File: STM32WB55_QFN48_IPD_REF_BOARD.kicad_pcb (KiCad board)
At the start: 4 copper layers, 72 parts, among them IC1 LD3985M33R, IC2 USBLC6-2SC6, J1 USB_B_Micro, J2 Conn_01x05_Male, J3 Conn_01x02_Male, J4 Conn_01x04_Male, J5 Conn_01x01_Male, J6 Conn_01x01_Male, J7 Conn_01x08_Male, U1 MCP1640CCH, U2 STM32WB55CG, U4 BNO055_my, U5 ADS1115IDGS, Y1 NX2520SA-32MHz, Y2 NX2012SA-32768K, Y3 NX2012SA-32768K

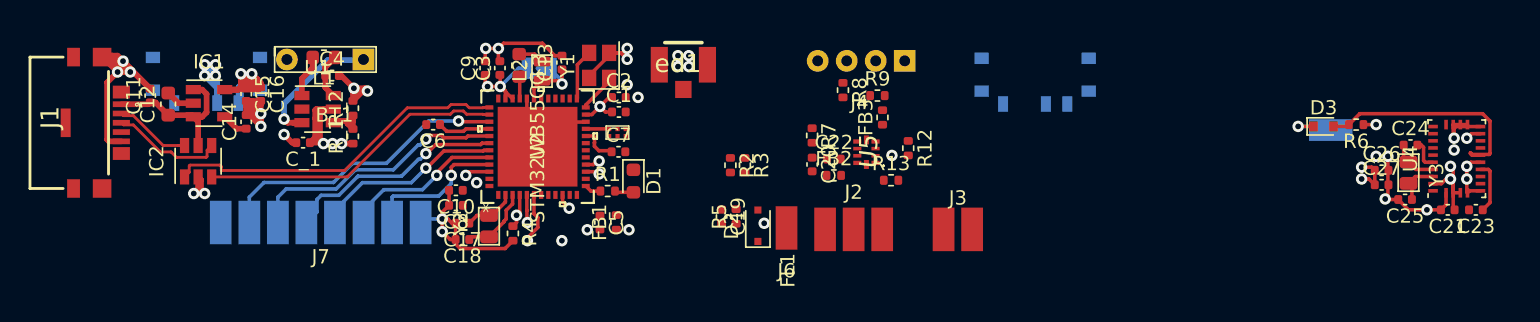
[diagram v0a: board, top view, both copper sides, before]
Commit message: v01
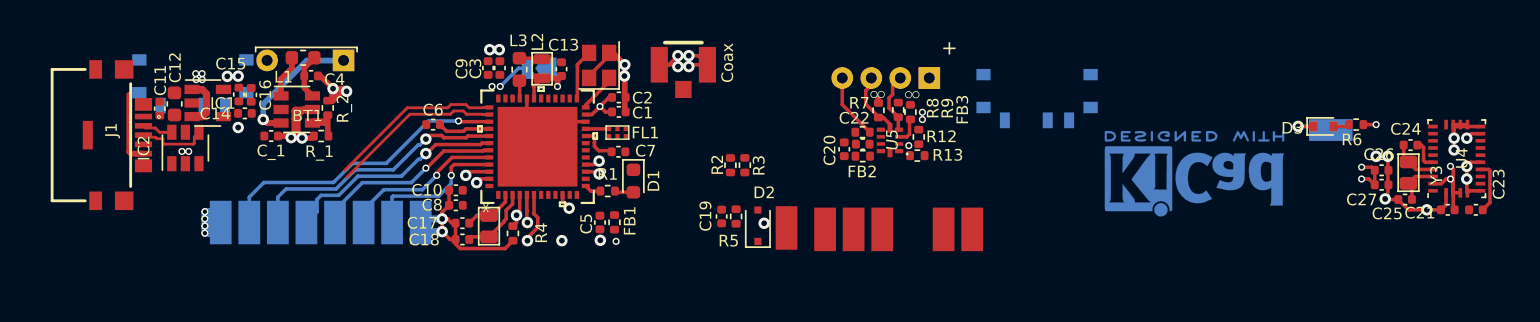
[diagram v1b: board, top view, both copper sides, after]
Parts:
- removed J3: Conn_01x02_Male, 0Pretty:pin_02
- removed J6: Conn_01x01_Male, 0Pretty:pin_01
- removed U1: MCP1640CCH, Package_TO_SOT_SMD:SOT-23-6
- added I2C: Conn_01x02_Male, 0Pretty:pin_02, F.Cu at (137.3, 113.6)
- added MCP: MCP1640CCH, Package_TO_SOT_SMD:SOT-23-6, F.Cu at (91.0, 105.2)
- added N1: Housing, Symbol:KiCad-Logo2_5mm_Copper, B.Cu at (153.9, 109.8)
- added NRSTR: Conn_01x01_Male, 0Pretty:pin_01, F.Cu at (125.3, 113.5)
- J7: moved to B.Cu
- U2: value STM32WB55CG -> STM32
- moved R7 3.54 mm to (130.7, 106.8), turned to 180 degrees
- moved R8 2.86 mm to (131.8, 105.3), turned to 90 degrees
- moved R13 2.52 mm to (134.5, 108.5)
- moved C20 2.49 mm to (129.4, 108.0)
- moved FB2 2.43 mm to (130.7, 108.5)
- moved C_1 2.28 mm to (89.2, 107.1)
- moved C22 2.28 mm to (130.7, 107.7)
- moved R_1 2.22 mm to (92.7, 107.1), turned to 0 degrees
- moved J4 2.10 mm to (133.2, 103.8)
- moved FB3 1.99 mm to (134.0, 105.4)
- moved BT1 1.89 mm to (91.7, 102.7)
- moved U5 1.85 mm to (132.6, 107.4)
- moved J1 1.77 mm to (79.4, 107.0)
- moved R9 1.77 mm to (133.2, 105.3), turned to 90 degrees
- moved R_2 1.76 mm to (93.2, 105.1)
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- renumbered Y2 to 32768K, Y1 to 32MHz, ed1 to Coax
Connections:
- U2 pad 49: (no net) -> GND
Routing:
- net GND: track 105.9 -> 69.7 mm, vias 31 -> 29
- net 3v3fromUSB: track 18.3 -> 0.00 mm, vias 2 -> 1
- net Net-(D3-Pad2): track 16.1 -> 1.13 mm
- net USB_D-: track 24.3 -> 12.2 mm
- net USB_D+: track 21.5 -> 12.0 mm
- net +5V: track 11.1 -> 3.40 mm
- net +3V3: track 36.7 -> 29.3 mm, vias 13 -> 19
- net Net-(J4-Pad4): track 0.00 -> 4.60 mm
- net Net-(J4-Pad3): track 0.00 -> 4.57 mm
- net Net-(J4-Pad2): track 0.00 -> 4.24 mm
- net USB_OD-: track 5.35 -> 2.17 mm
- net USB_OD+: track 7.93 -> 4.94 mm
- net 3v3fromBAT: track 11.6 -> 9.53 mm, vias 3 -> 2
- net Net-(FB3-Pad1): track 0.00 -> 1.87 mm
- net Net-(C14-Pad1): track 1.85 -> 0.00 mm
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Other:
- net class +3.3V added: clearance 0.2, trace_width 0.25, via_dia 0.5, via_drill 0.4
- net class GND added: clearance 0.2, trace_width 0.25, via_dia 0.5, via_drill 0.3
- net class USB Data added: clearance 0.2, trace_width 0.25, via_dia 0.8, via_drill 0.4
- board text added: "+"
